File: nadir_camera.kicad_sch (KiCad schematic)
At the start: 18 parts, among them J1 MOLEX_5051102491, U23 OPT4001, U5 BNO085, Y3 32.768kHz/12.5pF

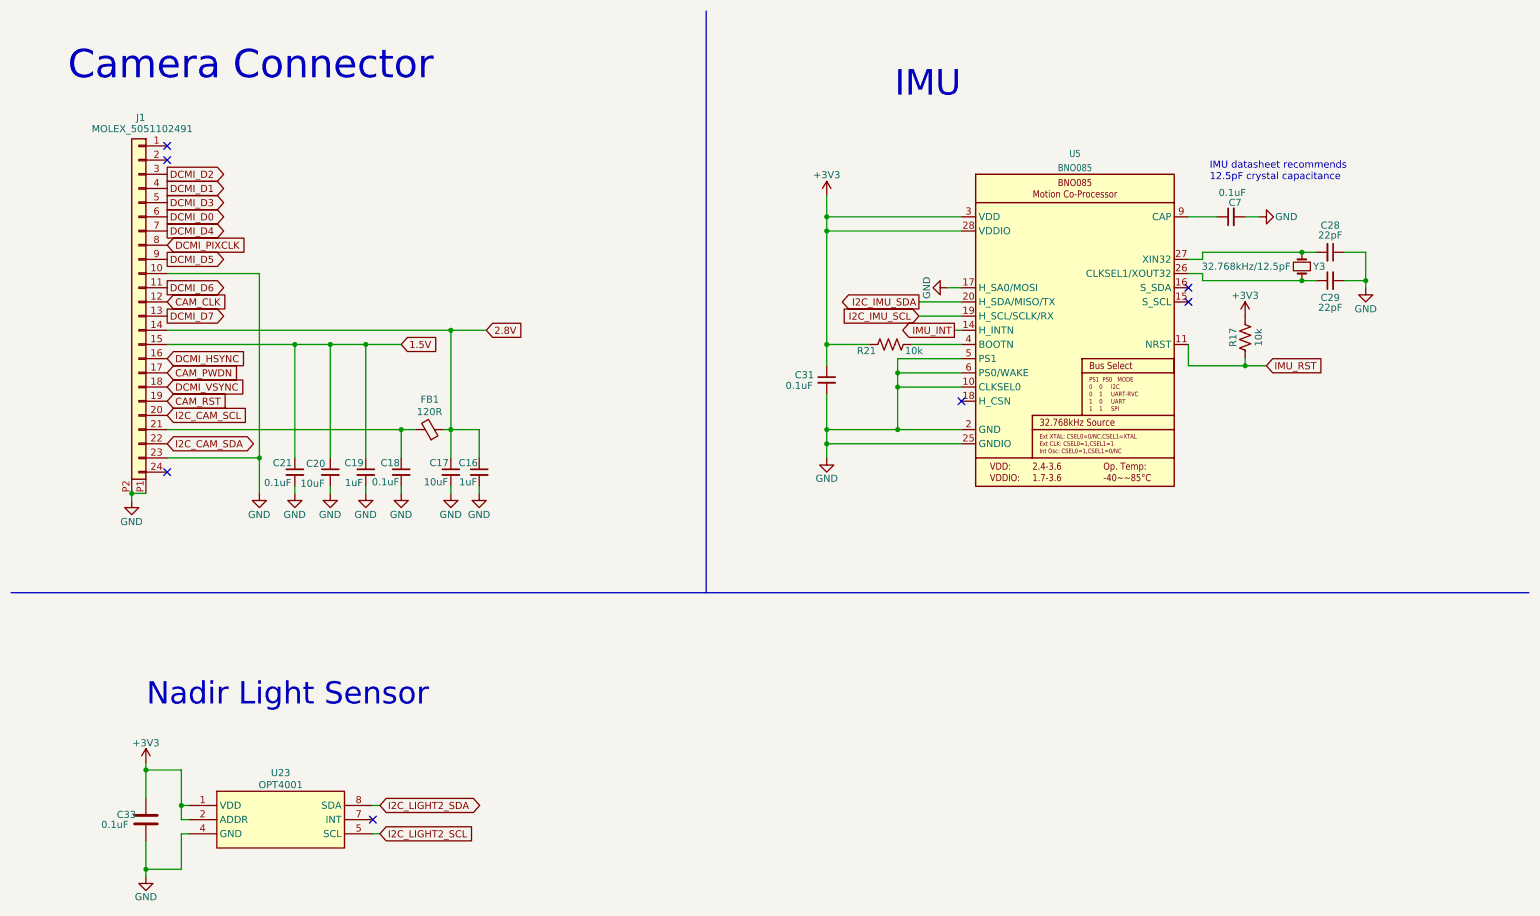
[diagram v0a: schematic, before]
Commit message: Move things around in schematic
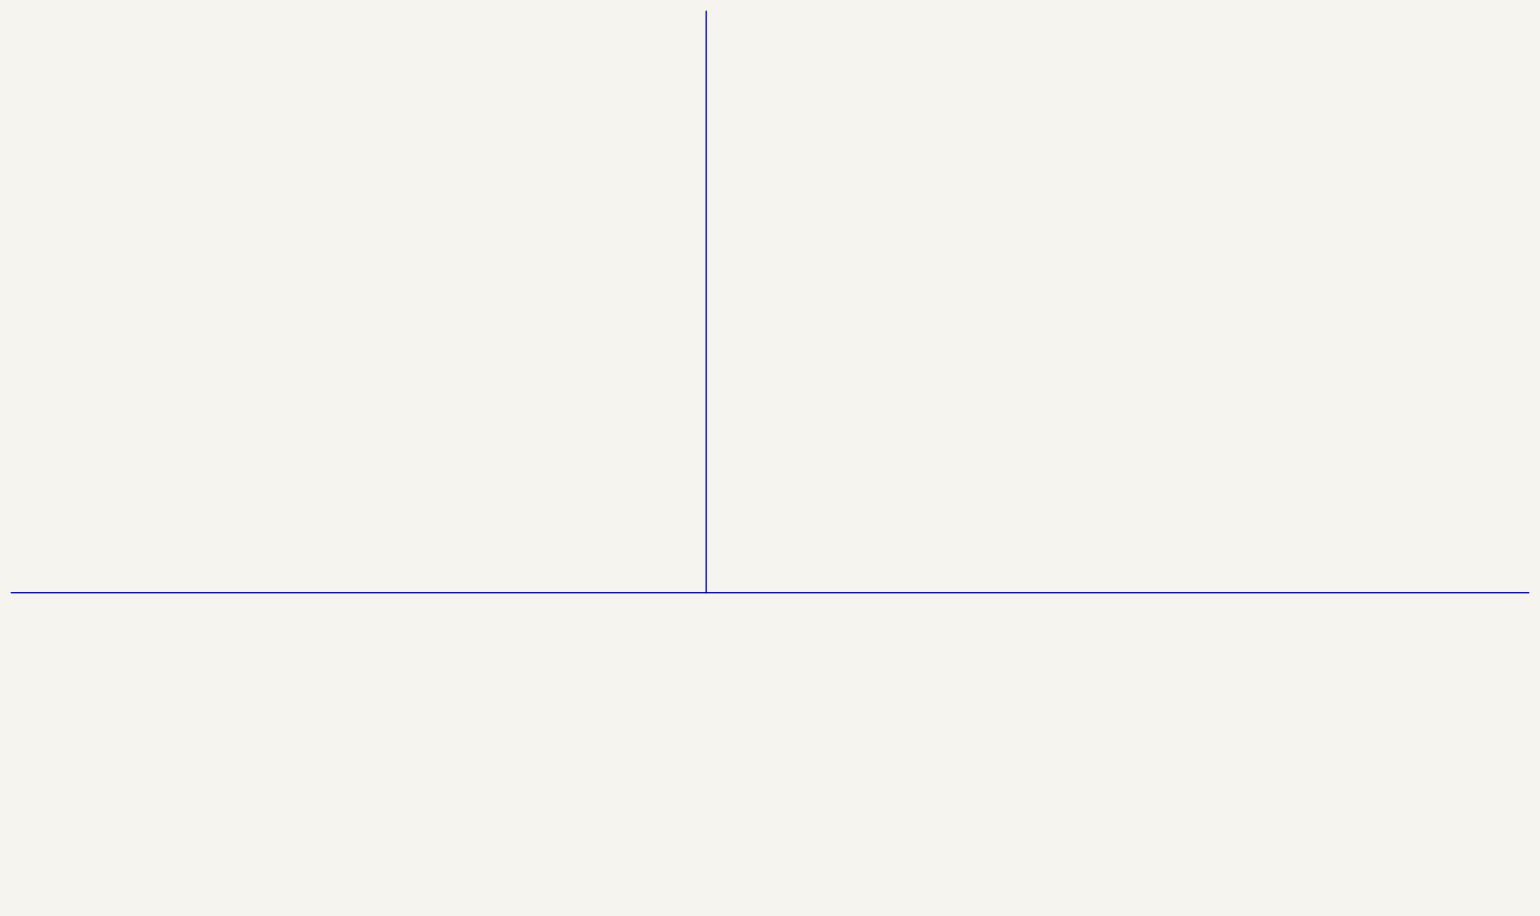
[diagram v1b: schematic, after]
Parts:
- removed C16, C19: 1uF, Capacitor_SMD:C_0603_1608Metric, symbol Device:C_Small
- removed C17, C20: 10uF, Capacitor_SMD:C_0603_1608Metric, symbol Device:C_Small
- removed C18, C21, C31, C7: 0.1uF, Capacitor_SMD:C_0603_1608Metric, symbol Device:C_Small
- removed C28, C29: 22pF, Capacitor_SMD:C_0603_1608Metric, symbol Device:C_Small
- removed C33: 0.1uF, Capacitor_SMD:C_0603_1608Metric, symbol Device:C
- removed FB1: 120R, Inductor_SMD:L_0603_1608Metric, symbol Device:FerriteBead_Small
- removed J1: MOLEX_5051102491, cameraboard:MOLEX_5051102491, symbol cameraboard:MOLEX_5051102491
- removed R17, R21: 10k, Resistor_SMD:R_0603_1608Metric, symbol Device:R_US
- removed U23: OPT4001, Package_TO_SOT_SMD:SOT-583-8, symbol solarpanels:OPT4001
- removed U5: BNO085, mainboard:BNO085, symbol mainboard:BNO085
- removed Y3: 32.768kHz/12.5pF, Crystal:Crystal_SMD_MicroCrystal_CC7V-T1A-2Pin_3.2x1.5mm, symbol Device:Crystal_Small
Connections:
- no-connect marks 7 -> 0
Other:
- note removed: "Camera Connector"
- note removed: "IMU"
- note removed: "IMU datasheet recommends 12.5pF crystal capacitance"
- note removed: "Nadir Light Sensor"
